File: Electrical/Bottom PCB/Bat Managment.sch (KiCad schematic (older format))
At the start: 15 parts, among them J301 Battery, SW301 SW_SPST, U301 MC78M05_TO252

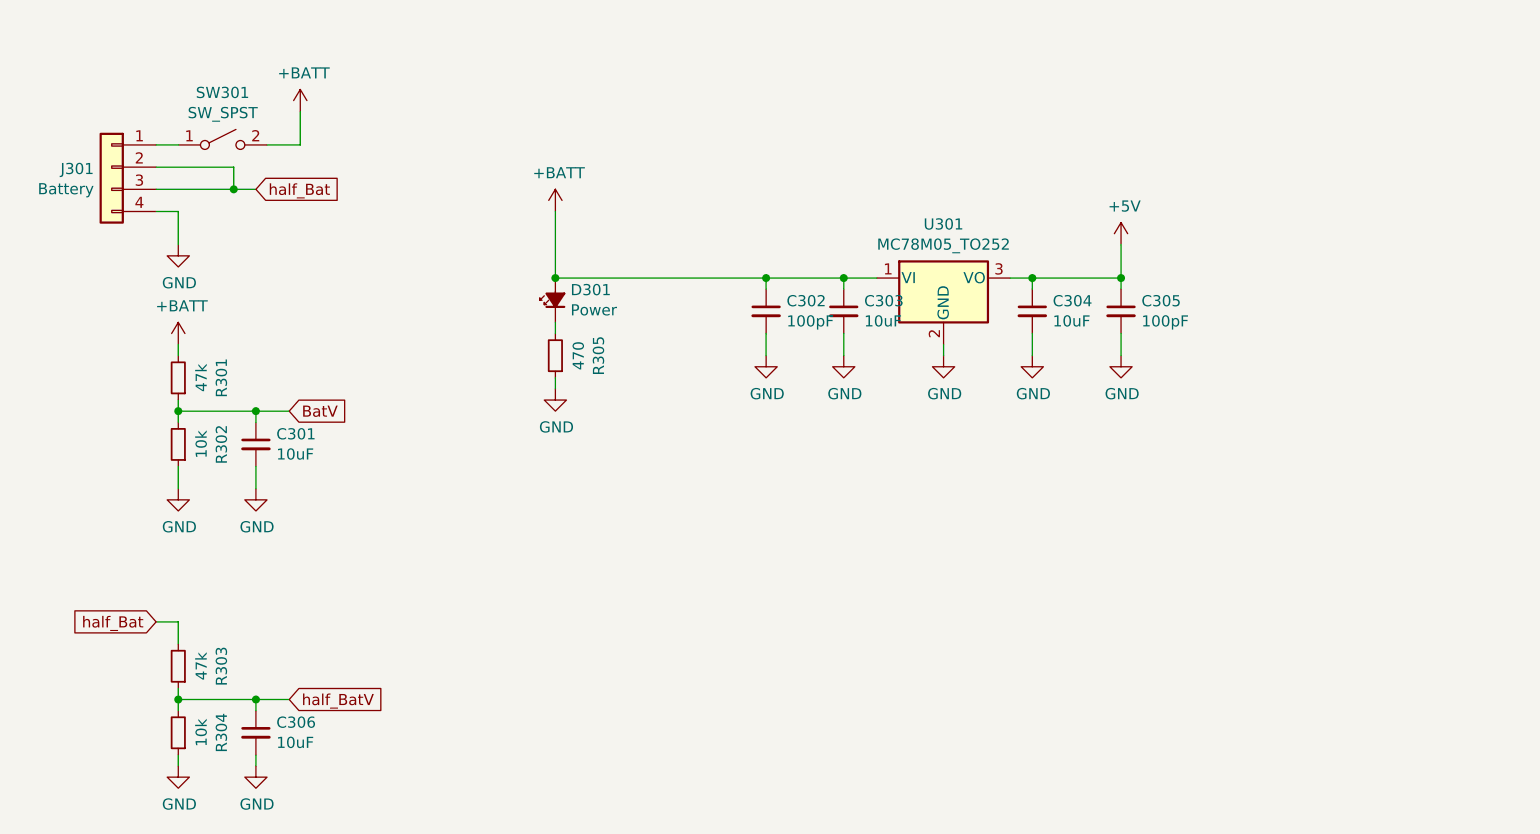
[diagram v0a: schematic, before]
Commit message: added more stuff
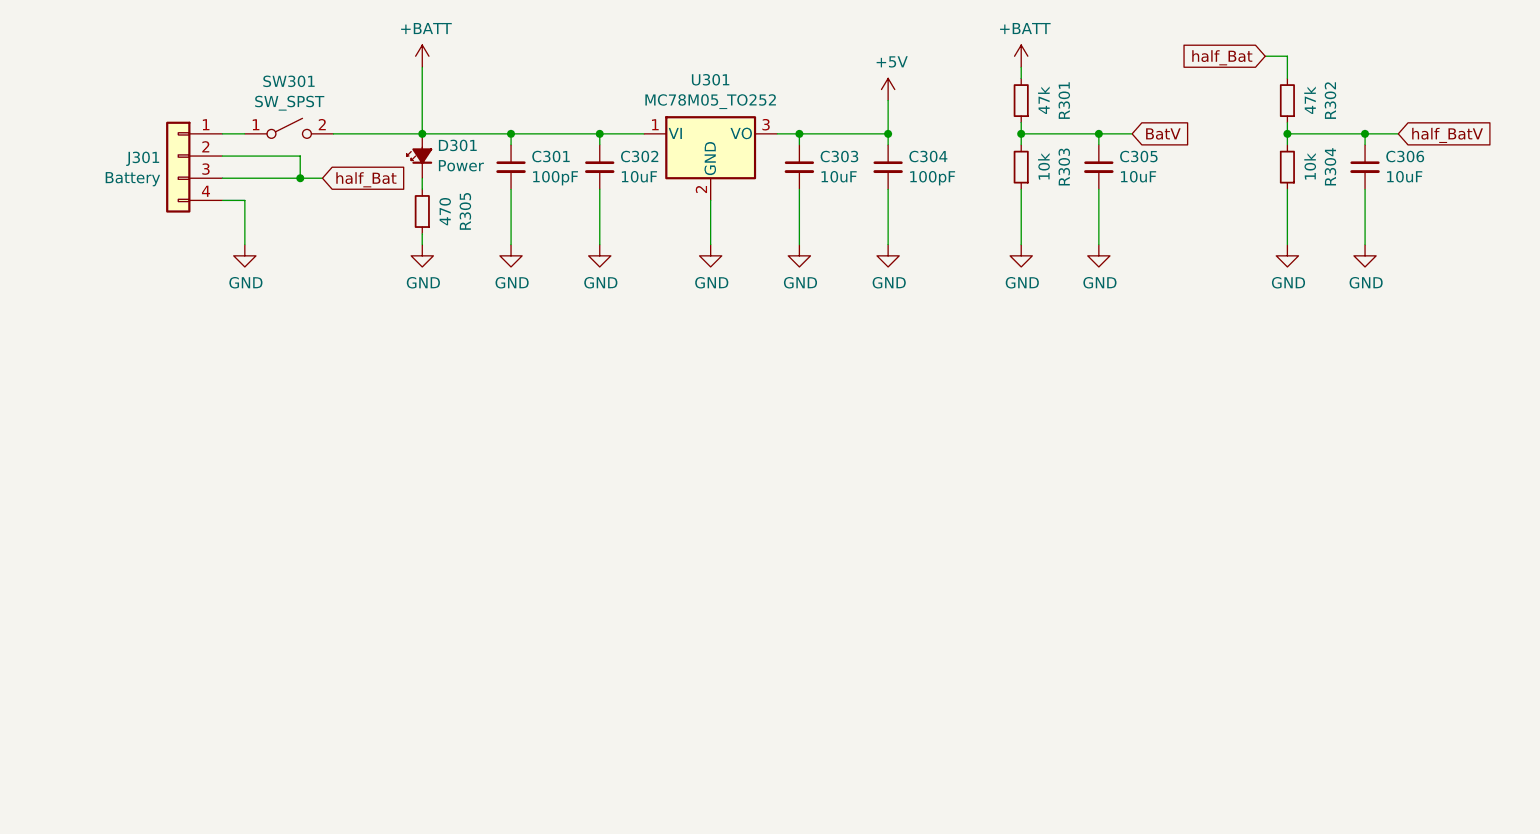
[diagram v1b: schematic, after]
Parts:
- renumbered C302 to C301, C303 to C302, C304 to C303, C305 to C304, C301 to C305, R303 to R302, R302 to R303
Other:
- moved on the sheet: C301, C302, C303, C304, C305, C306, D301, J301, R301, R302, R303, R304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
